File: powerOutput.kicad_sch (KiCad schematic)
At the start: 16 parts, among them J1 Screw_Terminal_01x02, J10 Screw_Terminal_01x04, J11 Screw_Terminal_01x04, J12 Screw_Terminal_01x04, J13 Conn_01x16_Pin, J9 Screw_Terminal_01x04, K1 SANYOU_SRD-S-124DM, K2 SANYOU_SRD-S-124DM, K3 SANYOU_SRD-S-124DM, K4 SANYOU_SRD-S-124DM, K5 SANYOU_SRD-S-124DM, K6 SANYOU_SRD-S-124DM, K7 SANYOU_SRD-S-124DM, K8 SANYOU_SRD-S-124DM, U4 ULN2803CDW, U7 ULN2803CDW

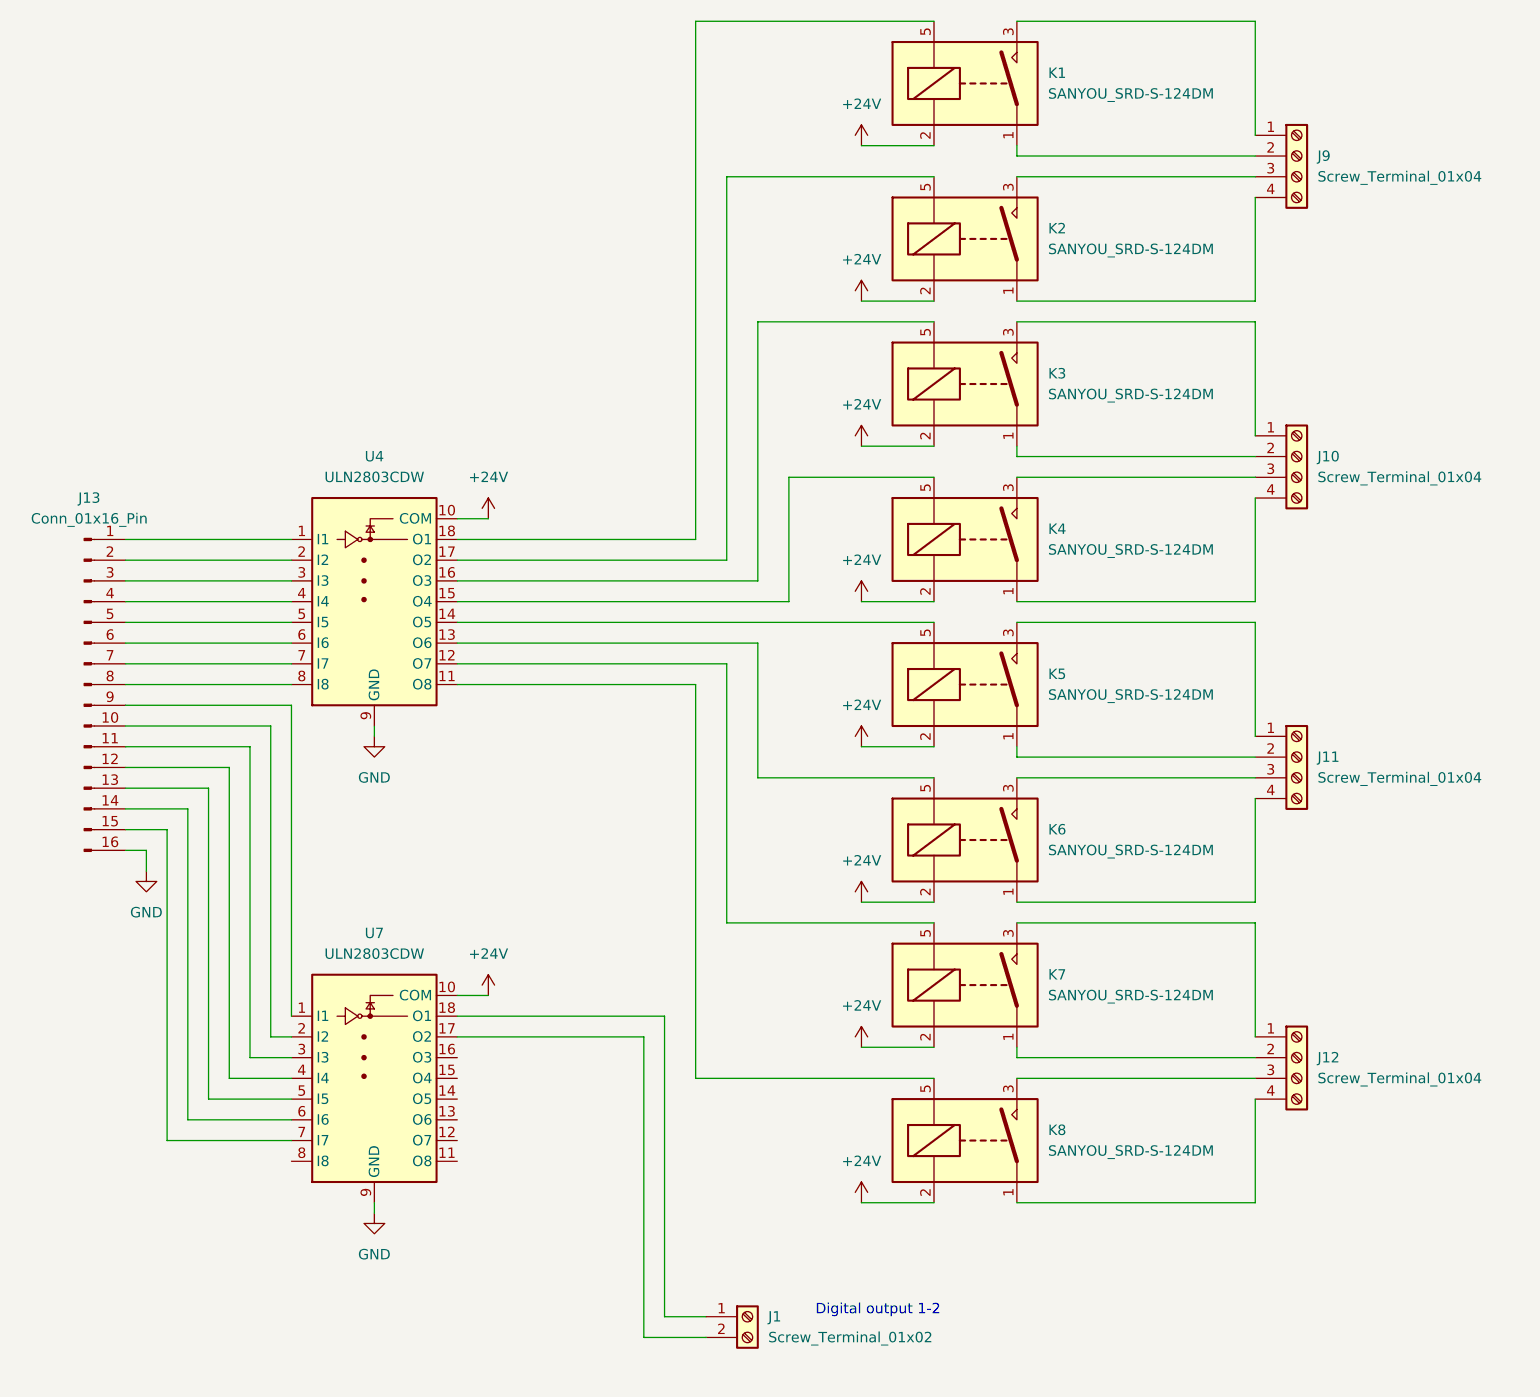
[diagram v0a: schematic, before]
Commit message: merged seperate projects
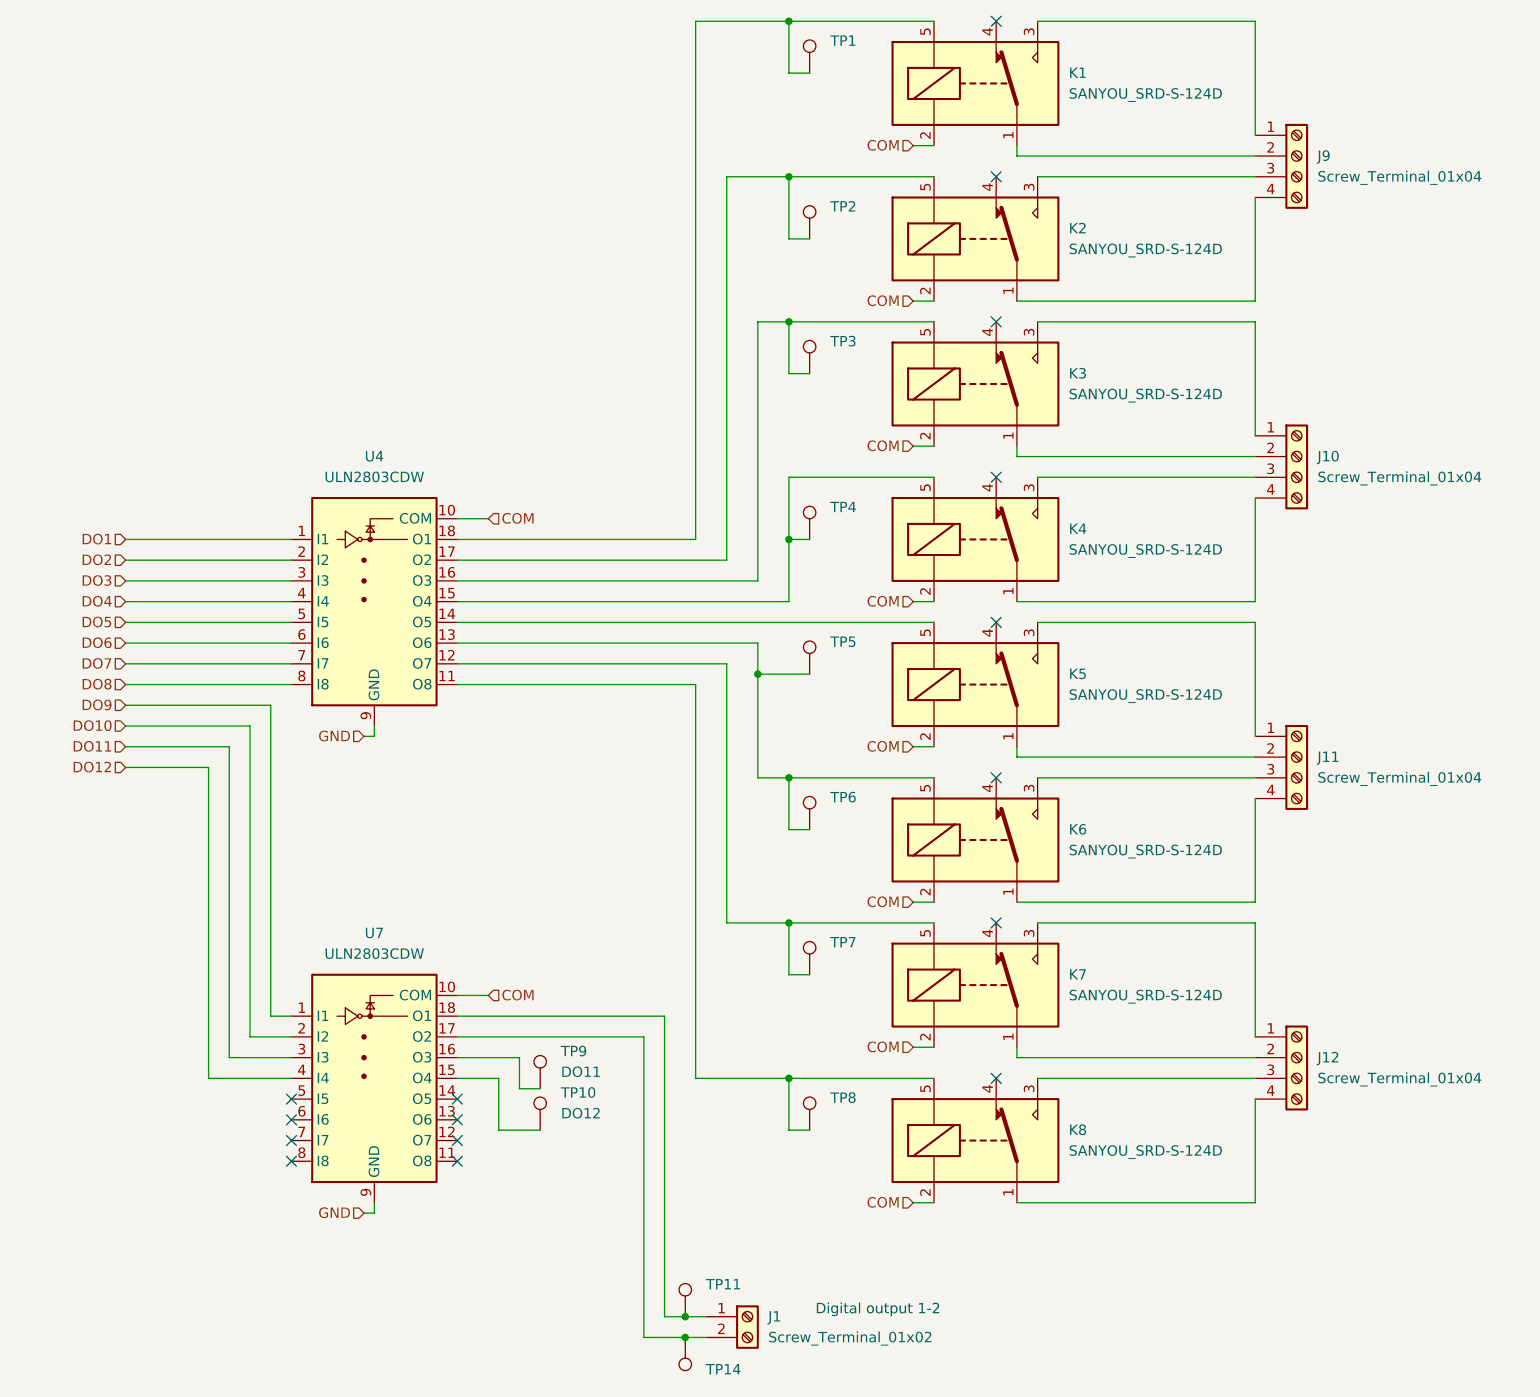
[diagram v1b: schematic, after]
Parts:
- removed J13: Conn_01x16_Pin, symbol Connector:Conn_01x16_Pin
- removed K1, K2, K3, K4, K5, K6, K7, K8: SANYOU_SRD-S-124DM, Relay_THT:Relay_SPST_SANYOU_SRD_Series_Form_A, symbol Relay:SANYOU_SRD_Form_A
- added K1, K2, K3, K4, K5, K6, K7, K8: SANYOU_SRD-S-124D, Relay_THT:Relay_SPDT_SANYOU_SRD_Series_Form_C, symbol Relay:SANYOU_SRD_Form_C
- added TP1, TP11, TP14, TP2, TP3, TP4, TP5, TP6, TP7, TP8: ~, symbol Connector:TestPoint
- added TP10: DO12, symbol Connector:TestPoint
- added TP9: DO11, symbol Connector:TestPoint
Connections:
- net at J11.1 (Pin_1): now also K5.3
- net at J11.2 (Pin_2): now also K5.1
- net at J11.3 (Pin_3): now also K6.3
- net at J11.4 (Pin_4): now also K6.1
- net at J12.4 (Pin_4): now also K8.1
- net at J12.3 (Pin_3): now also K8.3
- net at U4.11 (O8): now also K8.5, TP8.1
- net at J9.1 (Pin_1): now also K1.3
- net at J9.2 (Pin_2): now also K1.1
- net at J9.3 (Pin_3): now also K2.3
- net at J9.4 (Pin_4): now also K2.1
- net at J1.1 (Pin_1), U7.18 (O1): now also TP11.1
- net at J1.2 (Pin_2), U7.17 (O2): now also TP14.1
- net at U4.18 (O1): now also K1.5, TP1.1
- net at J10.4 (Pin_4): now also K4.1
- net at J10.3 (Pin_3): now also K4.3
- net at U4.15 (O4): now also K4.5, TP4.1
- net DO9: now reaches U7.1 (I1)
- net at U7.15 (O4): now also TP10.1
- net at U7.16 (O3): now also TP9.1
- net DO10: now reaches U7.2 (I2)
- net DO11: now reaches U7.3 (I3)
- net DO12: now reaches U7.4 (I4)
- net at U4.17 (O2): now also K2.5, TP2.1
- net at U4.14 (O5): now also K5.5
- net DO1: now reaches U4.1 (I1)
- net DO2: now reaches U4.2 (I2)
- net DO3: now reaches U4.3 (I3)
- net DO4: now reaches U4.4 (I4)
- net DO5: now reaches U4.5 (I5)
- net DO6: now reaches U4.6 (I6)
- net DO7: now reaches U4.7 (I7)
- net DO8: now reaches U4.8 (I8)
- net at J10.2 (Pin_2): now also K3.1
- net at J10.1 (Pin_1): now also K3.3
- net at U4.16 (O3): now also K3.5, TP3.1
- net at U4.13 (O6): now also K6.5, TP5.1, TP6.1
- net at J12.2 (Pin_2): now also K7.1
- net at J12.1 (Pin_1): now also K7.3
- net at U4.12 (O7): now also K7.5, TP7.1
- net +24V renamed COM
- net COM: now also K1.2, K2.2, K3.2, K4.2, K5.2, K6.2, K7.2, K8.2
- no-connect marks 0 -> 16

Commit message: added part numbers
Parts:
- J1: footprint (none) -> Connector_Phoenix_MC:PhoenixContact_MC_1,5_2-G-3.5_1x02_P3.50mm_Horizontal; LCSC (none) -> C61791
- J10, J11, J12, J9: footprint (none) -> Connector_Phoenix_MC:PhoenixContact_MC_1,5_4-G-3.5_1x04_P3.50mm_Horizontal; LCSC (none) -> C5241865
- K1, K2, K3, K4, K5, K6, K7, K8: LCSC (none) -> C276436
- U4, U7: footprint (none) -> Package_SO:SOIC-20W_7.5x12.8mm_P1.27mm; LCSC (none) -> C7494313
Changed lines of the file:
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@@
 			)
 		)
-		(property "Footprint" ""
+		(property "Footprint" "Connector_Phoenix_MC:PhoenixContact_MC_1,5_4-G-3.5_1x04_P3.50mm_Horizontal"
 			(at 168.91 104.14 0)
 			(effects
@@
 		)
 		(property "Description" "Generic screw terminal, single row, 01x04, script generated (kicad-library-utils/schlib/autogen/connector/)"
+			(at 168.91 104.14 0)
+			(effects
+				(font
+					(size 1.27 1.27)
+				)
+				(hide yes)
+			)
+		)
+		(property "LCSC" "C5241865"
 			(at 168.91 104.14 0)
 			(effects
@@
 			)
 		)
+		(property "LCSC" "C276436"
+			(at 129.54 21.59 0)
+			(effects
+				(font
+					(size 1.27 1.27)
+				)
+				(hide yes)
+			)
+		)
 		(pin "4"
 		)
@@
 			)
 		)
+		(property "LCSC" "C276436"
+			(at 129.54 151.13 0)
+			(effects
+				(font
+					(size 1.27 1.27)
+				)
+				(hide yes)
+			)
+		)
 		(pin "4"
 		)
@@
 			)
 		)
-		(property "Footprint" ""
+		(property "Footprint" "Connector_Phoenix_MC:PhoenixContact_MC_1,5_4-G-3.5_1x04_P3.50mm_Horizontal"
 			(at 168.91 30.48 0)
 			(effects
@@
 			)
 		)
+		(property "LCSC" "C5241865"
+			(at 168.91 30.48 0)
+			(effects
+				(font
+					(size 1.27 1.27)
+				)
+				(hide yes)
+			)
+		)
 		(pin "4"
 		)
@@
 			)
 		)
-		(property "Footprint" ""
+		(property "Footprint" "Connector_Phoenix_MC:PhoenixContact_MC_1,5_2-G-3.5_1x02_P3.50mm_Horizontal"
 			(at 101.6 172.72 0)
 			(effects
@@
 		)
 		(property "Description" "Generic screw terminal, single row, 01x02, script generated (kicad-library-utils/schlib/autogen/connector/)"
+			(at 101.6 172.72 0)
+			(effects
+				(font
+					(size 1.27 1.27)
+				)
+				(hide yes)
+			)
+		)
+		(property "LCSC" "C61791"
 			(at 101.6 172.72 0)
 			(effects
@@
 			)
 		)
+		(property "LCSC" "C276436"
+			(at 129.54 77.47 0)
+			(effects
+				(font
+					(size 1.27 1.27)
+				)
+				(hide yes)
+			)
+		)
 		(pin "4"
 		)
@@
 			)
 		)
+		(property "LCSC" "C276436"
+			(at 129.54 95.25 0)
+			(effects
+				(font
+					(size 1.27 1.27)
+				)
+				(hide yes)
+			)
+		)
 		(pin "4"
 		)
@@
 			)
 		)
-		(property "Footprint" ""
+		(property "Footprint" "Package_SO:SOIC-20W_7.5x12.8mm_P1.27mm"
 			(at 57.15 157.48 0)
 			(effects
@@
 		)
 		(property "Description" "Darlington Transistor Arrays, SOIC18/DIP18"
+			(at 55.88 140.97 0)
+			(effects
+				(font
+					(size 1.27 1.27)
+				)
+				(hide yes)
+			)
+		)
+		(property "LCSC" "C7494313"
 			(at 55.88 140.97 0)
 			(effects
@@
 			)
 		)
+		(property "LCSC" "C276436"
+			(at 129.54 132.08 0)
+			(effects
+				(font
+					(size 1.27 1.27)
+				)
+				(hide yes)
+			)
+		)
 		(pin "4"
 		)
@@
 			)
 		)
+		(property "LCSC" "C276436"
+			(at 129.54 40.64 0)
+			(effects
+				(font
+					(size 1.27 1.27)
+				)
+				(hide yes)
+			)
+		)
 		(pin "4"
 		)
@@
 			)
 		)
+		(property "LCSC" "C276436"
+			(at 129.54 114.3 0)
+			(effects
+				(font
+					(size 1.27 1.27)
+				)
+				(hide yes)
+			)
+		)
 		(pin "4"
 		)
@@
 			)
 		)
-		(property "Footprint" ""
+		(property "Footprint" "Connector_Phoenix_MC:PhoenixContact_MC_1,5_4-G-3.5_1x04_P3.50mm_Horizontal"
 			(at 168.91 67.31 0)
 			(effects
@@
 		)
 		(property "Description" "Generic screw terminal, single row, 01x04, script generated (kicad-library-utils/schlib/autogen/connector/)"
+			(at 168.91 67.31 0)
+			(effects
+				(font
+					(size 1.27 1.27)
+				)
+				(hide yes)
+			)
+		)
+		(property "LCSC" "C5241865"
 			(at 168.91 67.31 0)
 			(effects
@@
 			)
 		)
-		(property "Footprint" ""
+		(property "Footprint" "Connector_Phoenix_MC:PhoenixContact_MC_1,5_4-G-3.5_1x04_P3.50mm_Horizontal"
 			(at 168.91 140.97 0)
 			(effects
@@
 		)
 		(property "Description" "Generic screw terminal, single row, 01x04, script generated (kicad-library-utils/schlib/autogen/connector/)"
+			(at 168.91 140.97 0)
+			(effects
+				(font
+					(size 1.27 1.27)
+				)
+				(hide yes)
+			)
+		)
+		(property "LCSC" "C5241865"
 			(at 168.91 140.97 0)
 			(effects
@@
 			)
 		)
-		(property "Footprint" ""
+		(property "Footprint" "Package_SO:SOIC-20W_7.5x12.8mm_P1.27mm"
 			(at 57.15 99.06 0)
 			(effects
@@
 		)
 		(property "Description" "Darlington Transistor Arrays, SOIC18/DIP18"
+			(at 55.88 82.55 0)
+			(effects
+				(font
+					(size 1.27 1.27)
+				)
+				(hide yes)
+			)
+		)
+		(property "LCSC" "C7494313"
 			(at 55.88 82.55 0)
 			(effects
@@
 			(at 129.54 58.42 0)
 			(effects
+				(font
+					(size 1.27 1.27)
+				)
+				(hide yes)
+			)
+		)
+		(property "LCSC" "C276436"
+			(at 129.54 58.42 0)
+			(effects
